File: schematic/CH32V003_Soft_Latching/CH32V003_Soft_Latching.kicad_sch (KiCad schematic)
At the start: 13 parts, among them Q1 PMOS, Q2 NMOS, SW1 SW_Push, U1 CH32V003F4P6

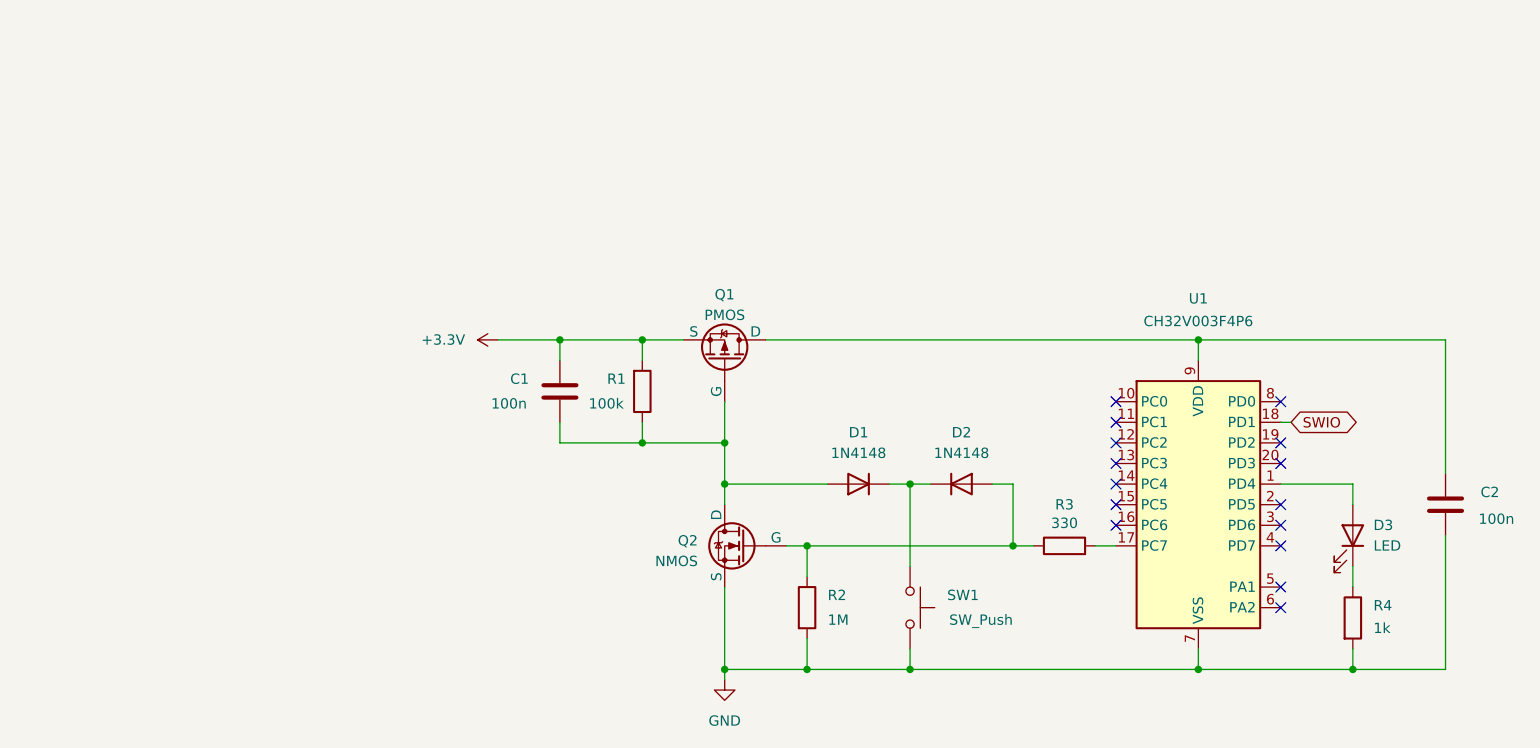
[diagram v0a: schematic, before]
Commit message: Update schematic
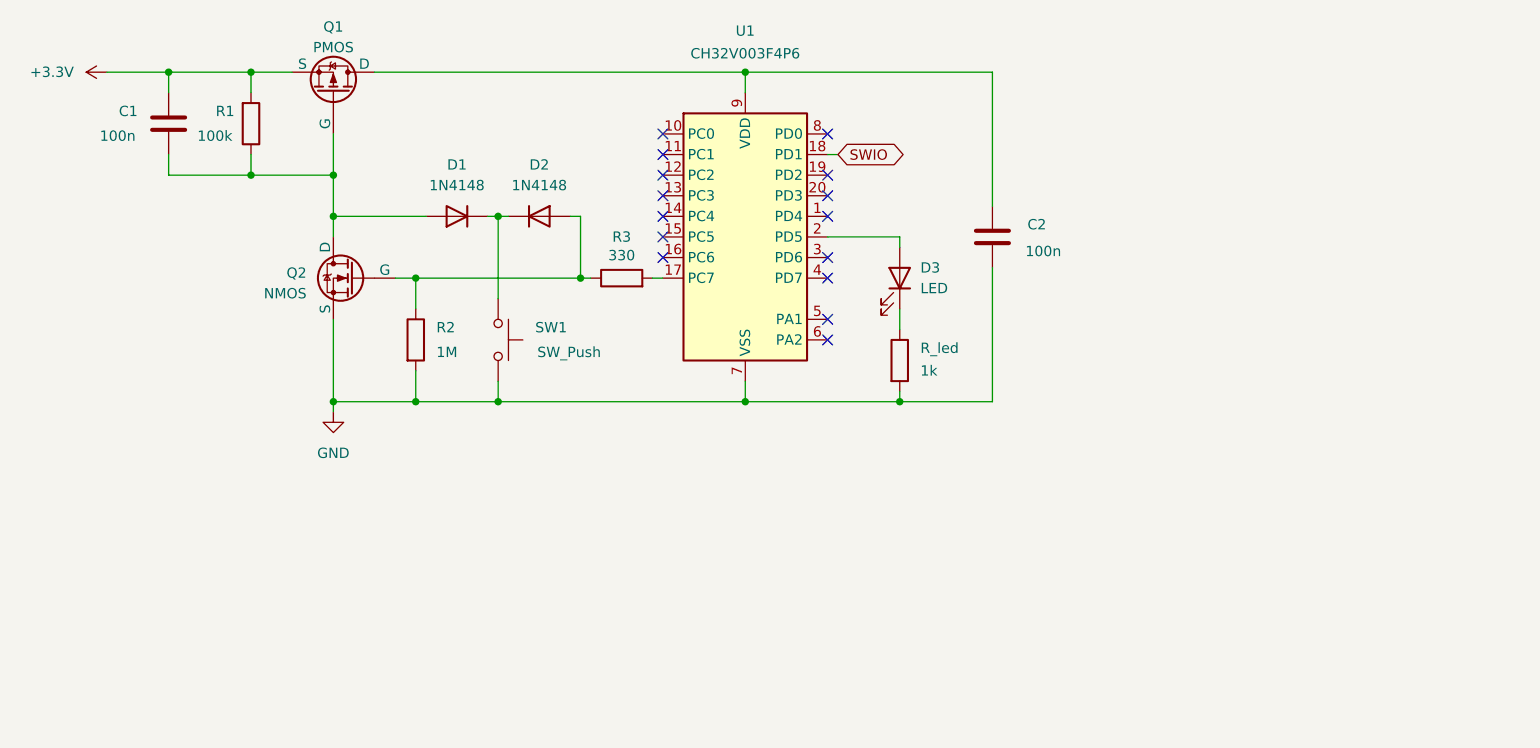
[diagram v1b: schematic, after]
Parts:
- renumbered R4 to R_led
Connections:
- net at U1.1 (PD4): no longer D3.2 (A)
- net at U1.2 (PD5): now also D3.2 (A)
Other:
- moved on the sheet: C1, C2, D1, D2, D3, Q1, Q2, R1, R2, R3, R_led, SW1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
